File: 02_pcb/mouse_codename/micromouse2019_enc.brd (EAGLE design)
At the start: 5.9 x 11.1 mm, 7 parts, among them IC1 AS5047D

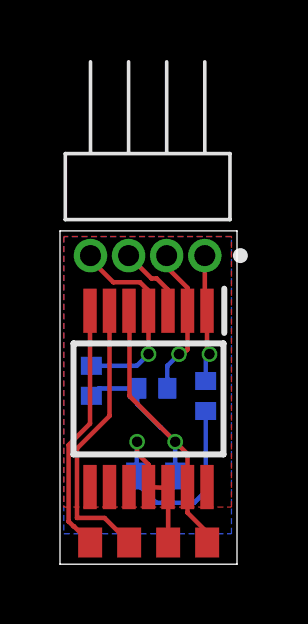
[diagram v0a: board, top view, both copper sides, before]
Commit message: module pcbs updated
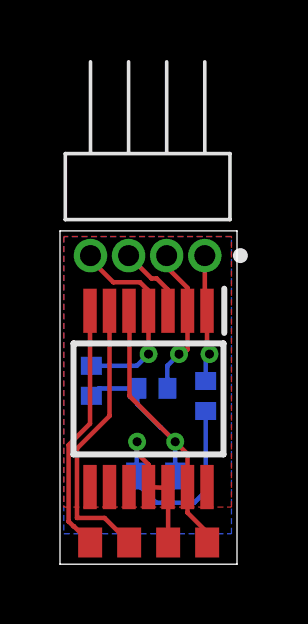
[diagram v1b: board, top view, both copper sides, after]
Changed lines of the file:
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@@
 <drawing>
 <settings>
-<setting alwaysvectorfont="yes"/>
+<setting alwaysvectorfont="no"/>
 <setting verticaltext="up"/>
 </settings>
-<grid distance="2.5" unitdist="mil" unit="mil" style="lines" multiple="1" display="yes" altdistance="0.1" altunitdist="mil" altunit="mil"/>
+<grid distance="2.5" unitdist="mil" unit="mm" style="lines" multiple="1" display="yes" altdistance="0.1" altunitdist="mil" altunit="mil"/>
 <layers>
 <layer number="1" name="Top" color="4" fill="1" visible="yes" active="yes"/>
@@
 <layer number="14" name="Route14" color="22" fill="1" visible="no" active="no"/>
 <layer number="15" name="Route15" color="23" fill="1" visible="no" active="no"/>
-<layer number="16" name="Bottom" color="1" fill="1" visible="no" active="yes"/>
+<layer number="16" name="Bottom" color="1" fill="1" visible="yes" active="yes"/>
 <layer number="17" name="Pads" color="2" fill="1" visible="yes" active="yes"/>
 <layer number="18" name="Vias" color="2" fill="1" visible="yes" active="yes"/>
@@
 <layer number="20" name="Dimension" color="24" fill="1" visible="yes" active="yes"/>
 <layer number="21" name="tPlace" color="7" fill="1" visible="yes" active="yes"/>
-<layer number="22" name="bPlace" color="7" fill="1" visible="no" active="yes"/>
+<layer number="22" name="bPlace" color="7" fill="1" visible="yes" active="yes"/>
 <layer number="23" name="tOrigins" color="15" fill="1" visible="yes" active="yes"/>
 <layer number="24" name="bOrigins" color="15" fill="1" visible="no" active="yes"/>
 <layer number="25" name="tNames" color="7" fill="1" visible="yes" active="yes"/>
-<layer number="26" name="bNames" color="7" fill="1" visible="no" active="yes"/>
+<layer number="26" name="bNames" color="7" fill="1" visible="yes" active="yes"/>
 <layer number="27" name="tValues" color="7" fill="1" visible="yes" active="yes"/>
 <layer number="28" name="bValues" color="7" fill="1" visible="no" active="yes"/>
@@
 <dimension x1="2.95" y1="5.51" x2="0" y2="5.51" x3="1.475" y3="23.41" textsize="1.778" layer="47" dtype="horizontal" width="0.05" extwidth="0.01" extlength="2" precision="3"/>
 <dimension x1="5.9" y1="0" x2="5.9" y2="11.11" x3="11.58" y3="5.555" textsize="1.778" layer="47" dtype="horizontal" width="0.05" extwidth="0.01" extlength="2" precision="3"/>
-<text x="2.6289" y="7.0866" size="0.7112" layer="26" rot="R90">MISO</text>
-<text x="1.3589" y="7.0993" size="0.7112" layer="26" rot="R90">MOSI</text>
+<text x="2.5019" y="6.8326" size="0.8128" layer="26" rot="R90">MISO</text>
+<text x="1.4224" y="6.8453" size="0.8128" layer="26" rot="R90">MOSI</text>
 <text x="3.8989" y="7.6962" size="0.7112" layer="28" rot="R90">CLK</text>
-<text x="5.1689" y="7.5184" size="0.7112" layer="26" rot="R90">CSN</text>
+<text x="5.2324" y="7.2644" size="0.8128" layer="26" rot="R90">CSN</text>
+<text x="3.1115" y="7.3025" size="0.8128" layer="26" rot="MR90">CLK</text>
 </plain>
 <attributes>
@@
 <wire x1="2.9510375" y1="3.32058125" x2="2.5700375" y2="3.70158125" width="0.1524" layer="1"/>
 <wire x1="2.5700375" y1="3.70158125" x2="2.5700375" y2="4.08258125" width="0.1524" layer="1"/>
-<via x="2.5700375" y="4.08258125" extent="1-16" drill="0.35"/>
+<via x="2.5700375" y="4.08258125" extent="1-16" drill="0.3" diameter="0.6"/>
 <wire x1="2.5700375" y1="4.08258125" x2="2.5550375" y2="4.06758125" width="0.1524" layer="16"/>
 <wire x1="2.5550375" y1="4.06758125" x2="2.5550375" y2="2.93958125" width="0.1524" layer="16"/>
@@
 <wire x1="4.2510375" y1="7.16058125" x2="4.0940375" y2="7.00358125" width="0.1524" layer="1"/>
 <wire x1="4.0940375" y1="7.00358125" x2="3.9670375" y2="7.00358125" width="0.1524" layer="1"/>
-<via x="3.9670375" y="7.00358125" extent="1-16" drill="0.35"/>
+<via x="3.9670375" y="7.00358125" extent="1-16" drill="0.3" diameter="0.6"/>
 <wire x1="3.5780375" y1="5.86058125" x2="3.5780375" y2="6.61458125" width="0.1524" layer="16"/>
 <wire x1="3.5780375" y1="6.61458125" x2="3.9670375" y2="7.00358125" width="0.1524" layer="16"/>
@@
 <wire x1="2.3160375" y1="5.60658125" x2="2.3160375" y2="8.40258125" width="0.1524" layer="1"/>
 <wire x1="2.3160375" y1="8.40258125" x2="2.3" y2="8.448" width="0.1524" layer="1"/>
-<via x="3.8400375" y="4.08258125" extent="1-16" drill="0.35"/>
+<via x="3.8400375" y="4.08258125" extent="1-16" drill="0.3" diameter="0.6"/>
 <wire x1="2.5780375" y1="5.86058125" x2="1.2920375" y2="5.86058125" width="0.1524" layer="16"/>
 <wire x1="1.0460375" y1="5.61458125" x2="1.2920375" y2="5.86058125" width="0.1524" layer="16"/>
@@
 <wire x1="4.9" y1="8.448" x2="4.9010375" y2="7.08558125" width="0.1524" layer="1"/>
 <wire x1="4.9010375" y1="7.08558125" x2="4.9830375" y2="7.00358125" width="0.1524" layer="1"/>
-<via x="4.9830375" y="7.00358125" extent="1-16" drill="0.35"/>
+<via x="4.9830375" y="7.00358125" extent="1-16" drill="0.3" diameter="0.6"/>
 <wire x1="4.9830375" y1="7.00358125" x2="4.8560375" y2="6.87658125" width="0.1524" layer="16"/>
 <wire x1="4.8560375" y1="6.87658125" x2="4.8560375" y2="6.10658125" width="0.1524" layer="16"/>
@@
 <contactref element="R3" pad="2"/>
 <wire x1="2.95" y1="8.448" x2="2.9510375" y2="7.00358125" width="0.1524" layer="1"/>
-<via x="2.9510375" y="7.00358125" extent="1-16" drill="0.35"/>
+<via x="2.9510375" y="7.00358125" extent="1-16" drill="0.3" diameter="0.6"/>
 <wire x1="2.9510375" y1="7.00358125" x2="2.5620375" y2="6.61458125" width="0.1524" layer="16"/>
 <wire x1="2.5620375" y1="6.61458125" x2="1.0460375" y2="6.61458125" width="0.1524" layer="16"/>
